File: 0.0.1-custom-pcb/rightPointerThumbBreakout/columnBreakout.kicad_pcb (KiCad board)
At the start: 2 copper layers, 42.5 x 63.3 mm, 21 parts, among them J1 HC-FPC-0.5-14P-FH20, J10 HC-FPC-0.5-6P-FH20, J11 HC-FPC-0.5-6P-FH20, J12 HC-FPC-0.5-6P-FH20, J13 HC-FPC-0.5-6P-FH20, J14 HC-FPC-0.5-6P-FH20, J15 HC-FPC-0.5-6P-FH20, J16 HC-FPC-0.5-6P-FH20, J17 HC-FPC-0.5-6P-FH20, J2 HC-FPC-0.5-6P-FH20, J3 HC-FPC-0.5-6P-FH20, J4 HC-FPC-0.5-6P-FH20, J5 HC-FPC-0.5-6P-FH20, J6 HC-FPC-0.5-6P-FH20, J7 HC-FPC-0.5-6P-FH20, J8 HC-FPC-0.5-6P-FH20, J9 HC-FPC-0.5-6P-FH20

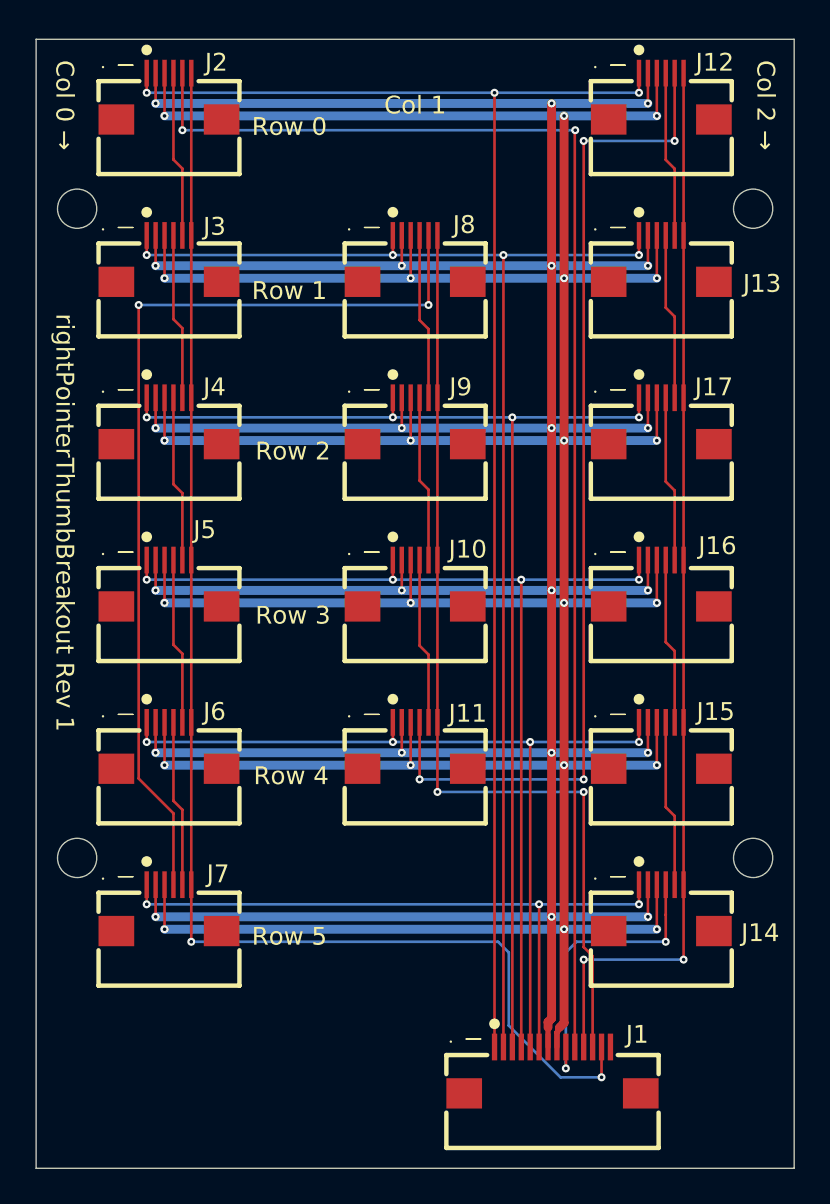
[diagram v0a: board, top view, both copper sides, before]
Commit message: right pointerThumb ready for order
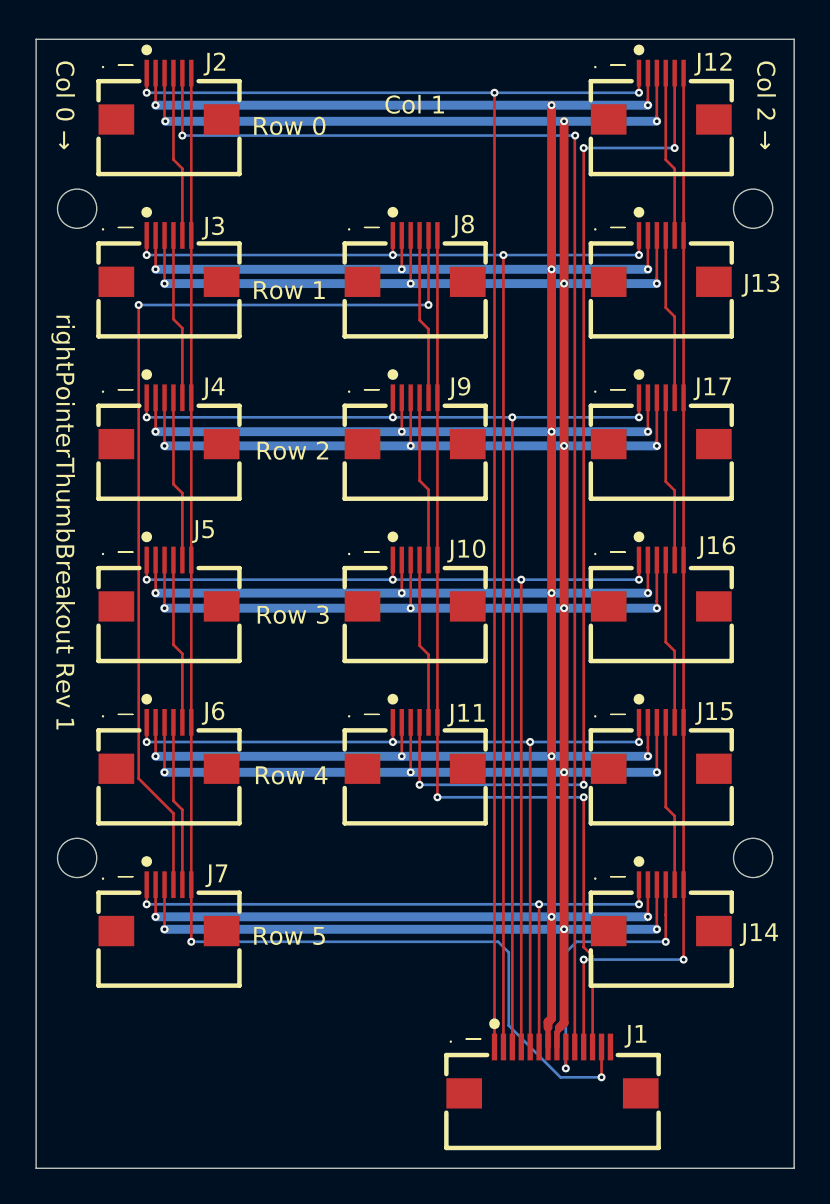
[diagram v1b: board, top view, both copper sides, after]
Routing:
- net /GND: track 256.7 -> 260.8 mm
- net /VDD: track 246.0 -> 248.4 mm
- net /IN10: track 57.1 -> 57.7 mm
